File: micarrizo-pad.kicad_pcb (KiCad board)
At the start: 2 copper layers, 128.6 x 81.8 mm, 20 parts, among them U1 The-Big-Switch, U2 KB2040

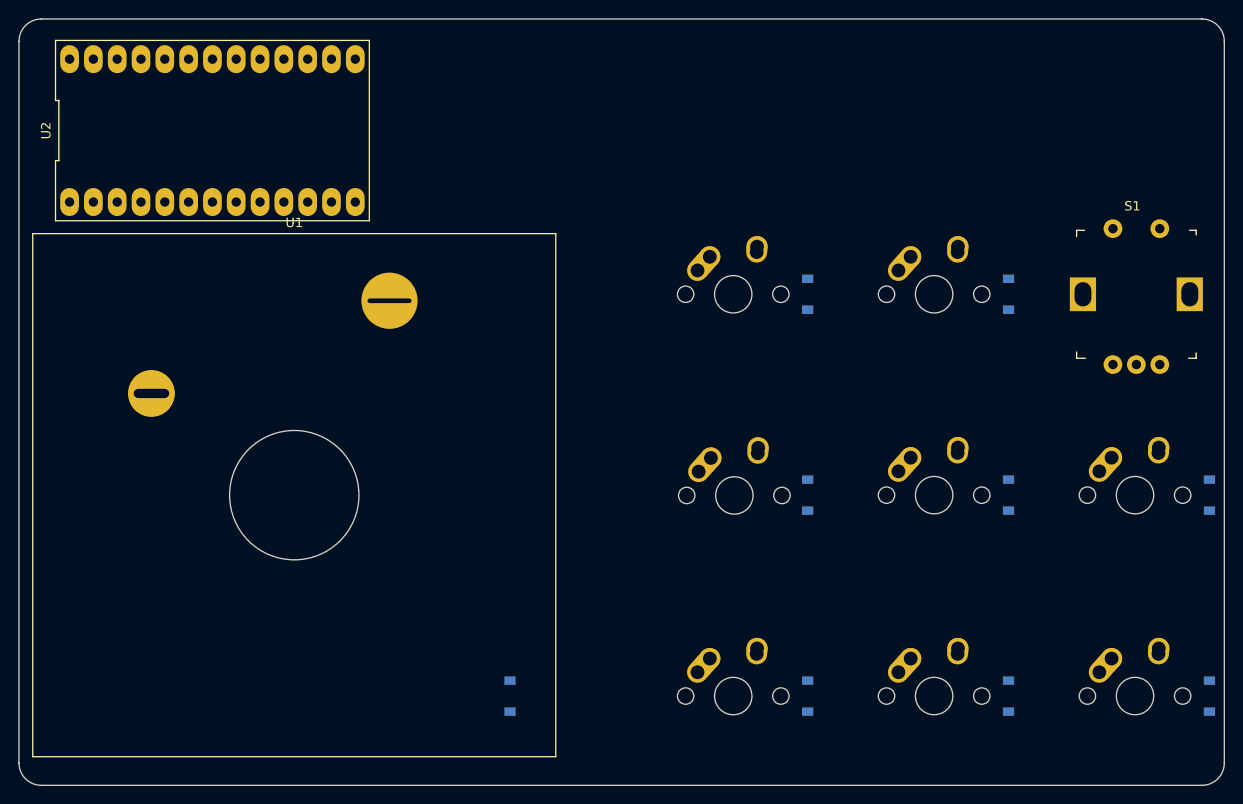
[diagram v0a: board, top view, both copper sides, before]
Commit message: finish pcb
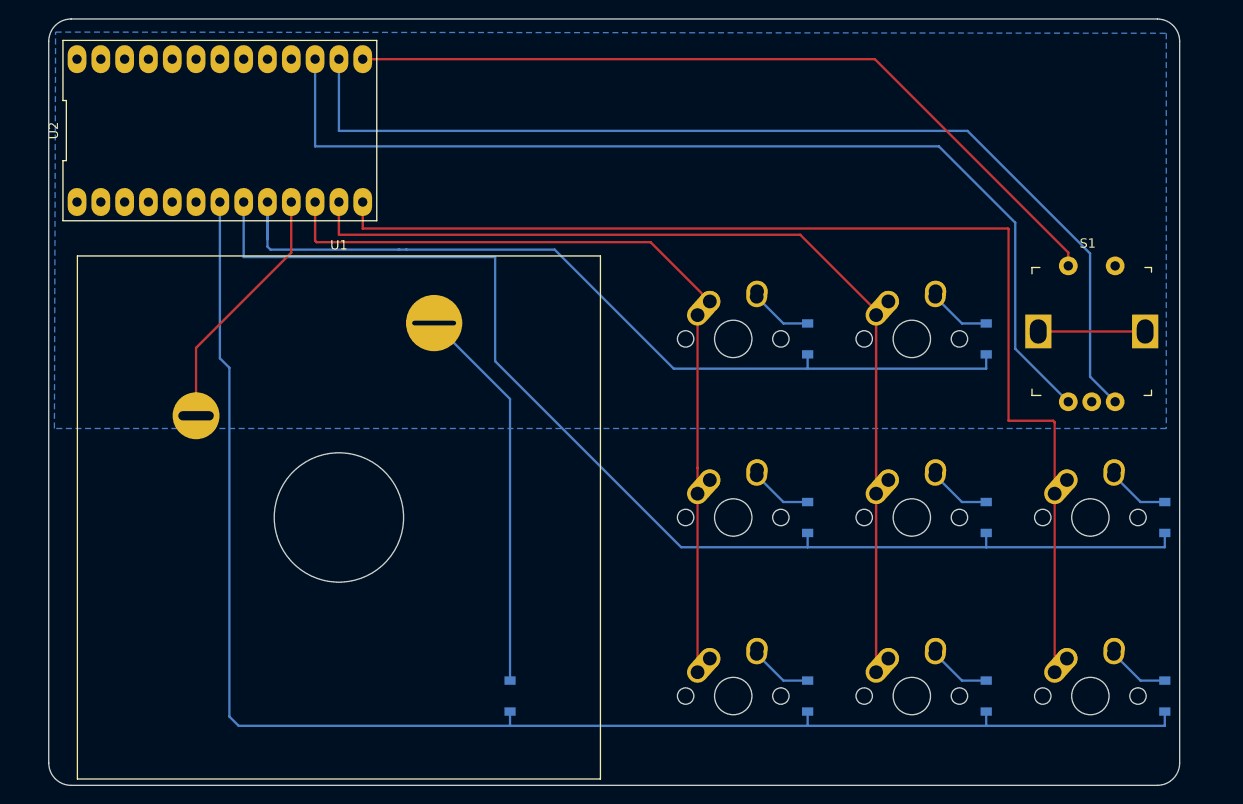
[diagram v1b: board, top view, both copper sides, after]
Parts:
- moved S1 6.20 mm to (134.9, 65.1)
- moved U1 5.32 mm to (60.3, 84.9)
- moved MX2 5.32 mm to (121.4, 65.9)
- moved D2 5.32 mm to (129.4, 65.9)
- moved D5 5.32 mm to (148.4, 84.9)
- moved MX5 5.32 mm to (140.5, 84.9)
- moved D1 4.76 mm to (110.3, 65.9)
- moved MX1 4.76 mm to (102.4, 65.9)
- moved D9 4.76 mm to (148.4, 104.0)
- moved MX8 4.76 mm to (140.5, 104.0)
- moved MX4 3.37 mm to (121.4, 84.9)
- moved D4 3.37 mm to (129.4, 84.9)
- moved D3 2.38 mm to (110.3, 84.9)
- moved MX7 2.38 mm to (121.4, 104.0)
- moved D8 2.38 mm to (129.4, 104.0)
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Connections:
- U2 pad 10: COL1 -> COL0
- U2 pad 11: COL2 -> COL1
- U2 pad 12: COL3 -> COL2
- U2 pad 13: COL4 -> COL3
- U2 pad 20: ENC_A -> Net-(U2-Pad20)
- U2 pad 21: ENC_B -> Net-(U2-Pad21)
- U2 pad 22: ENC_SW -> Net-(U2-Pad22)
- U2 pad 24: Net-(U2-Pad24) -> ENC_A
- U2 pad 25: Net-(U2-Pad25) -> ENC_B
- U2 pad 26: Net-(U2-Pad26) -> ENC_SW
- U2 pad 7: ROW1 -> ROW2
- U2 pad 8: ROW2 -> ROW1
- U2 pad 9: ROW3 -> ROW0
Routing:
- net ROW2: track 0.00 -> 161.6 mm
- net ROW1: track 0.00 -> 128.0 mm
- net COL3: track 0.00 -> 123.9 mm
- net ENC_B: track 0.00 -> 110.1 mm
- net ENC_A: track 0.00 -> 108.8 mm
- net COL2: track 0.00 -> 102.7 mm
- net ROW0: track 0.00 -> 94.1 mm
- net COL1: track 0.00 -> 87.0 mm
- net ENC_SW: track 0.00 -> 85.2 mm
- net Net-(D6-Pad2): track 0.00 -> 41.5 mm
- net COL0: track 0.00 -> 27.0 mm
- net Net-(S1-Pad3): track 0.00 -> 11.4 mm
- net Net-(D2-Pad2): track 0.00 -> 6.62 mm
- net Net-(D1-Pad2): track 0.00 -> 6.62 mm
- net Net-(D9-Pad2): track 0.00 -> 6.62 mm
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- added copper zone on B.Cu, net GND
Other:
- board size 128.6 x 81.8 mm -> 120.7 x 81.8 mm
